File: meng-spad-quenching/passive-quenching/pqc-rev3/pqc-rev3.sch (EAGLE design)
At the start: 62 parts, among them IC1 TPS7A4901, IC2 OPA858, IC3 OPA858, IC4 LM8261, Q1 NTR5105P, Q2 BSS123LT1G, Q3 NUD3160LT1G, X1 VIN_BIAS, X2 SPAD, X3 SIGNAL_OUT, X4 VIN_PWR

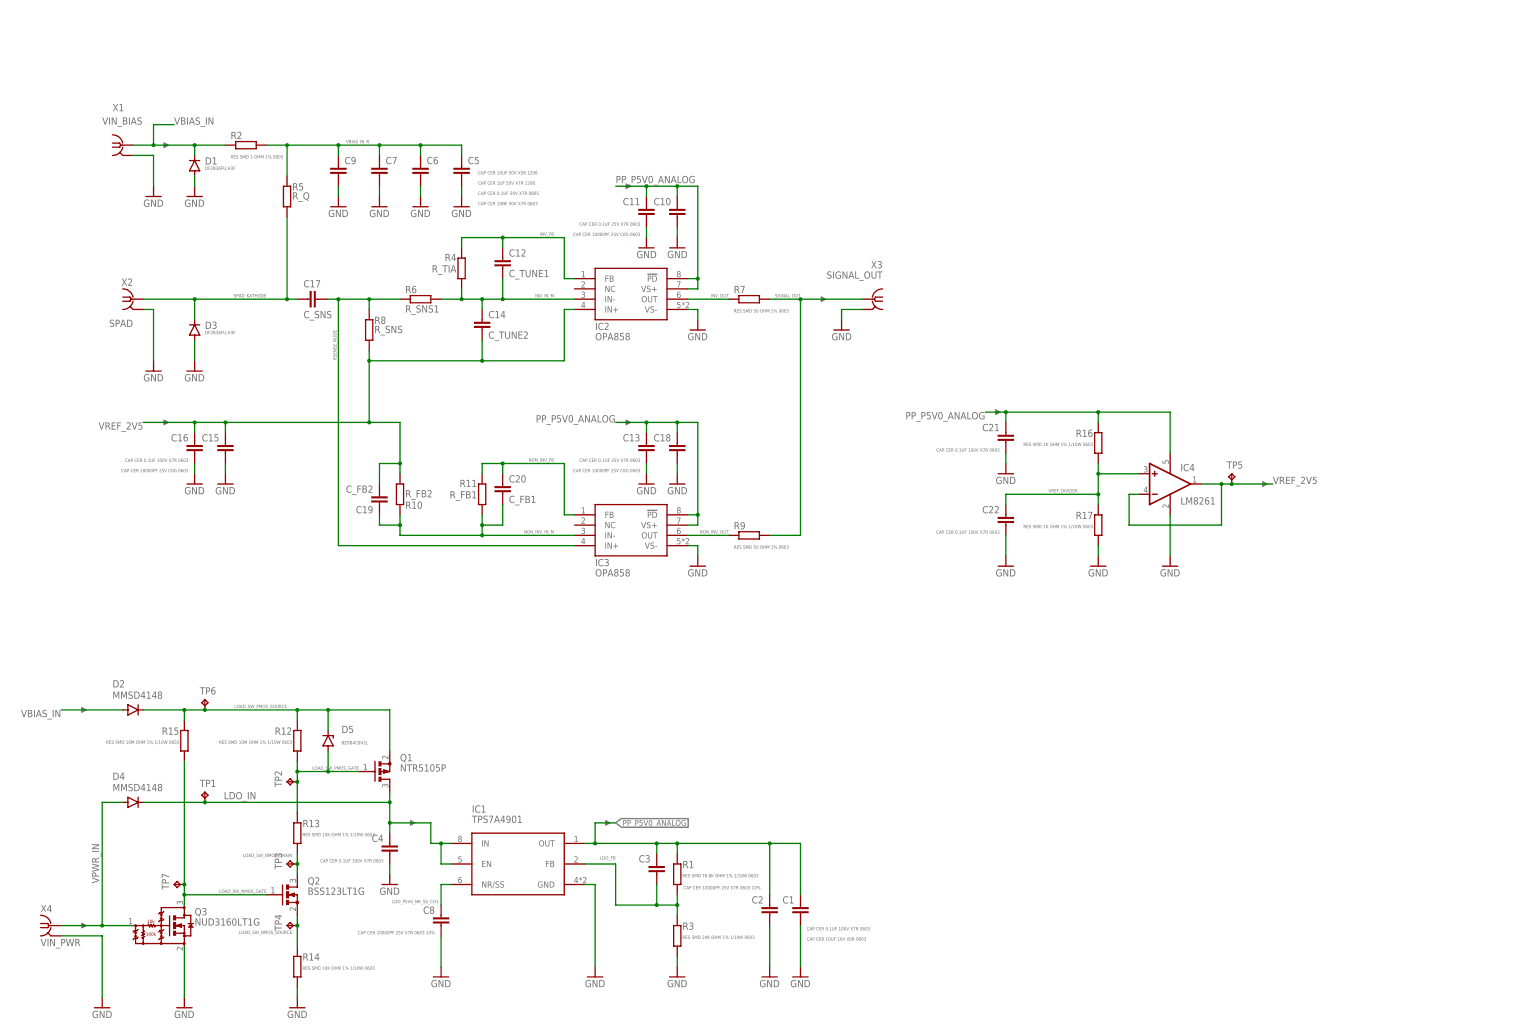
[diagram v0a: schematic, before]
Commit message: Fixed filenames
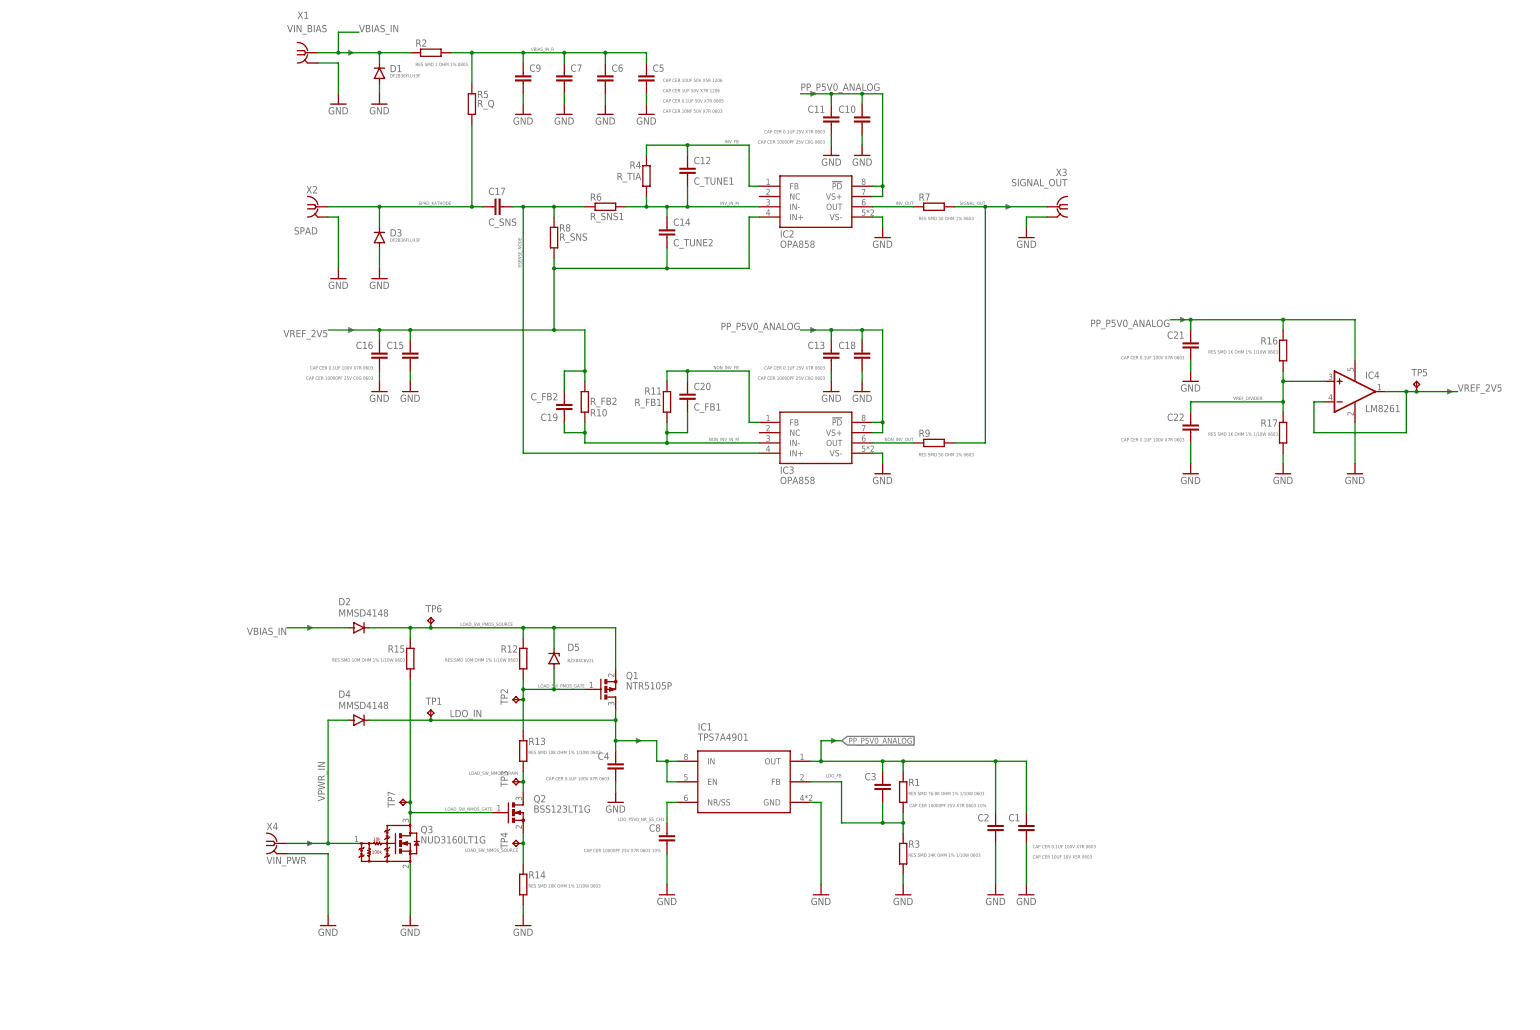
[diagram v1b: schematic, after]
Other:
- moved on the sheet: C1, C10, C11, C12, C13, C14, C15, C16, C17, C18, C19, C2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

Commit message: work on BOMs
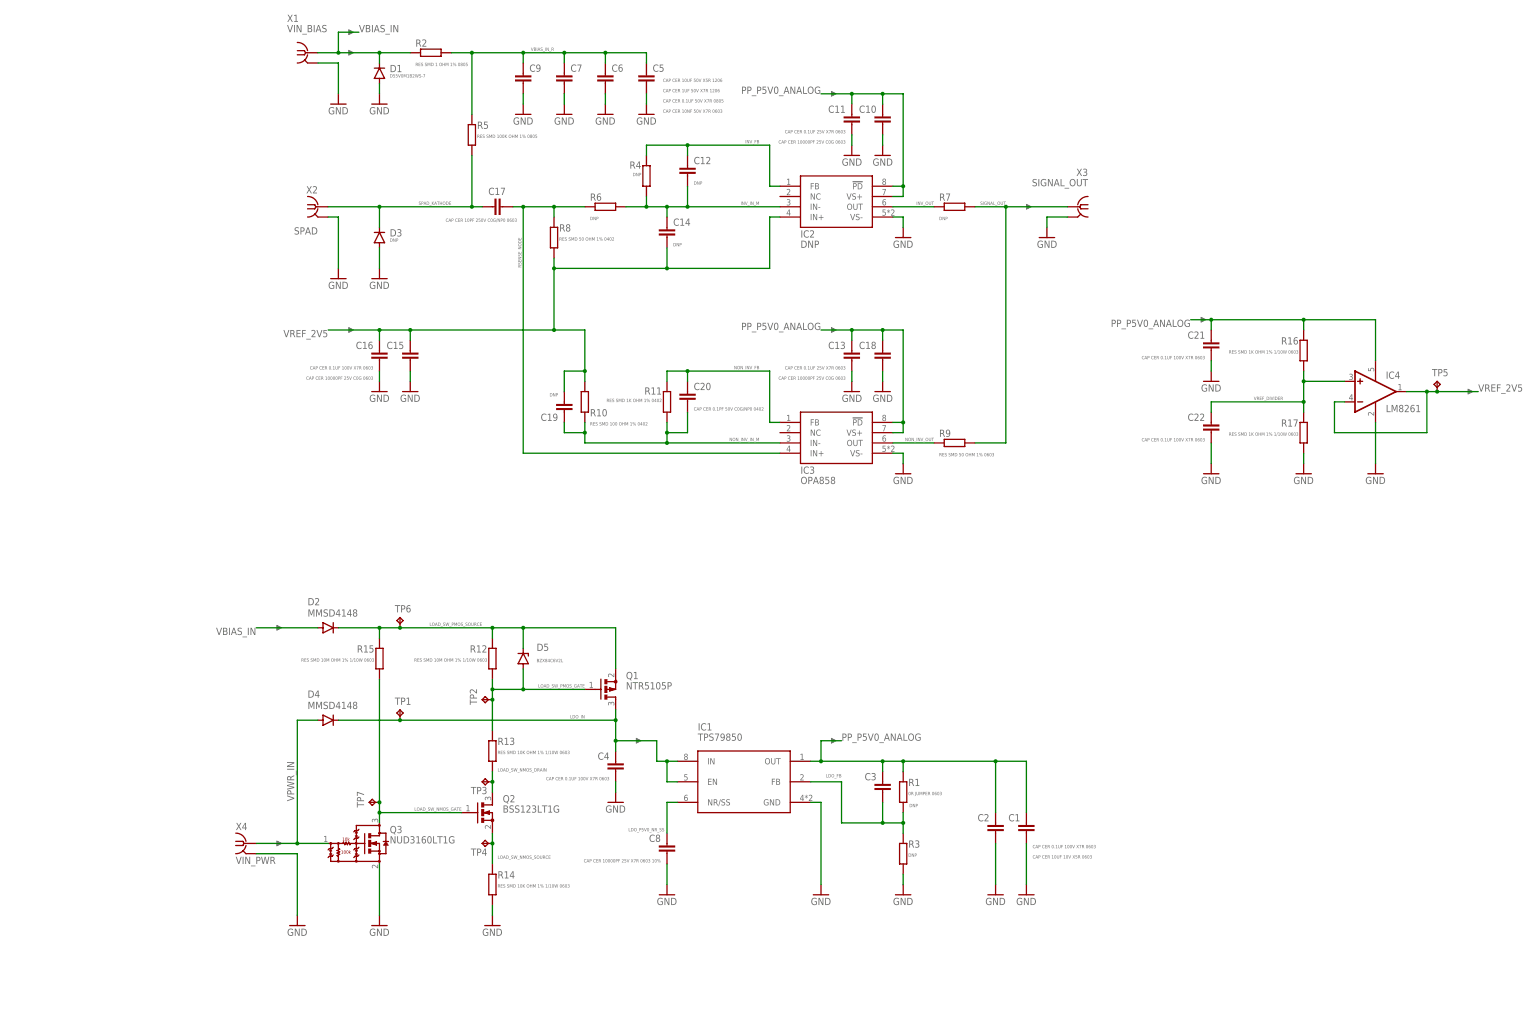
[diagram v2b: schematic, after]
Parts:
- C12: value C_TUNE1 -> DNP
- C14: value C_TUNE2 -> DNP
- C17: value C_SNS -> CAP CER 10PF 250V C0G/NP0 0603
- C19: value C_FB2 -> DNP
- C20: value C_FB1 -> CAP CER 0.1PF 50V C0G/NP0 0402
- C3: value CAP CER 10000PF 25V X7R 0603 10% -> DNP
- D1: value DF2B36FU,H3F -> D55V0M1B2WS-7
- D3: value DF2B36FU,H3F -> DNP
- IC1: value TPS7A4901 -> TPS79850
- IC2: value OPA858 -> DNP
- R1: value RES SMD 76.8K OHM 1% 1/10W 0603 -> 0R JUMPER 0603
- R10: value R_FB2 -> RES SMD 100 OHM 1% 0402
- R11: value R_FB1 -> RES SMD 1K OHM 1% 0402
- R3: value RES SMD 24K OHM 1% 1/10W 0603 -> DNP
- R4: value R_TIA -> DNP
- R5: value R_Q -> RES SMD 100K OHM 1% 0805
- R6: value R_SNS1 -> DNP
- R7: value RES SMD 50 OHM 1% 0603 -> DNP
- R8: value R_SNS -> RES SMD 50 OHM 1% 0402
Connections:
- net LDO_P5V0_NR_SS_CH1 renamed LDO_P5V0_NR_SS
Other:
- note added: "Compensation Cap (RF/Hi-Q)"
- note added: "ESD 55V standoff, 57V breakdown (min), 100V clamping (max)"
- note added: "Midrail reference buffer Stable under any cap load"
- note added: "Quench Resistor"
- note added: "Sense Resistor"
- note added: "Signal Coupling Cap (RF/Hi-Q)"
- note added: "TPS7A4901: R1 = 76.8K C3 = 10nF C3 = 24K Vout = 5V"
- note added: "This package pinout works for various MSOP8 Power Pad high-voltage LDOs. Checked: LT3010-5 (10k-100k = 100uVrms noise) TPS79850 (10k-100k = 100uVrms noise) TPS7A4901 (35V MAX INPUT!)"
- note removed: "ESD Update MPN for 50V"
- note removed: "Midrail reference buffer"
- note removed: "This package pinout works for various MSOP8 Power Pad high-voltage LDOs. Checked: LT3010-5 (10k-100k = 100uVrms noise) TPS79850 (10k-100k = 100uVrms noise)"
- moved on the sheet: C10, C11, C13, C18, C21, C22, C8, D2, D4, D5, IC2, IC3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
